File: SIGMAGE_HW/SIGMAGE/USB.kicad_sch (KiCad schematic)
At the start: 27 parts, among them J1 UJ31CHG2SMTTR, U13 ESDR0502NMUTBG, U9 FT2232HLTRAY

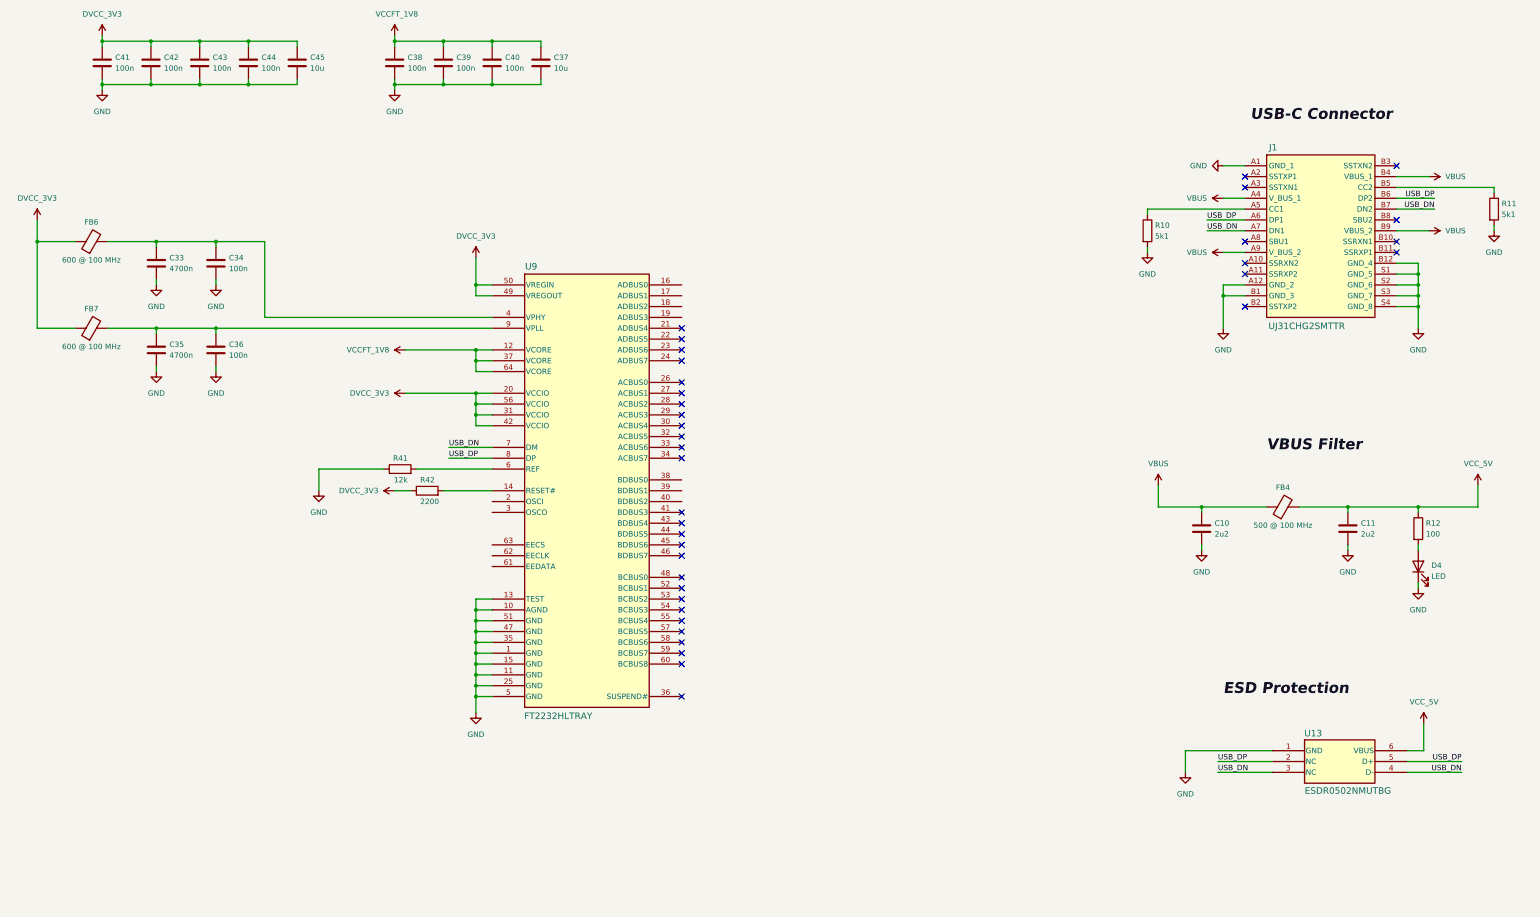
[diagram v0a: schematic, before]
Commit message: more USB stuff
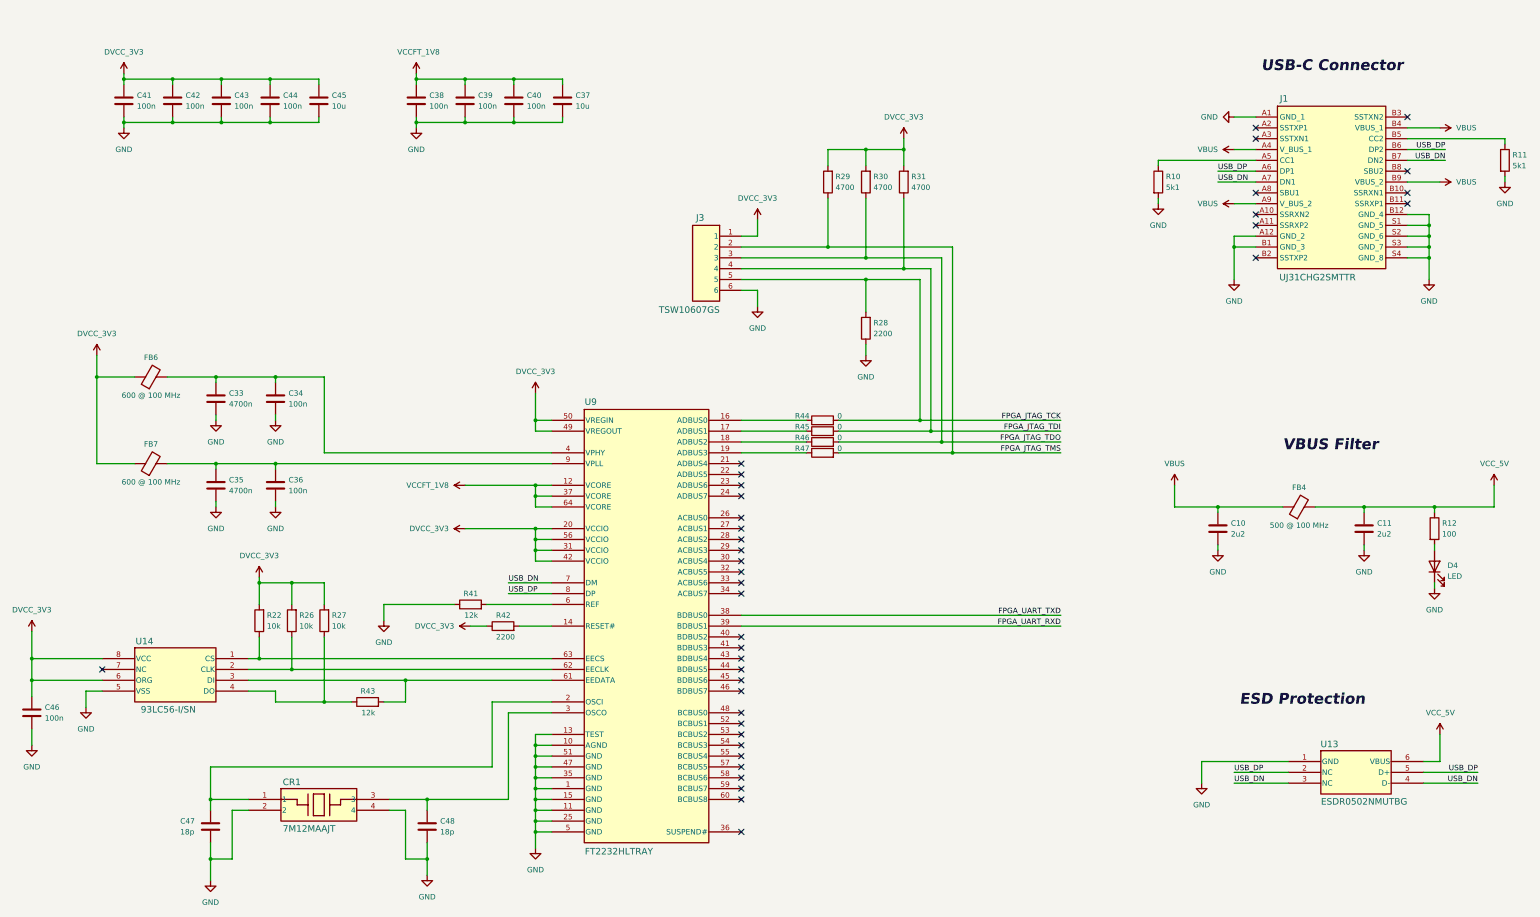
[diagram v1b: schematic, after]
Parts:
- added C46: 100n, Capacitor_SMD:C_0603_1608Metric, symbol Device:C
- added C47, C48: 18p, Capacitor_SMD:C_0603_1608Metric, symbol Device:C
- added CR1: 7M12MAAJT, SIGMAGE:7M12MAAJT, symbol SIGMAGE:7M12MAAJT
- added J3: TSW10607GS, SIGMAGE:TSW10607GS, symbol SIGMAGE:TSW10607GS
- added R22, R26, R27: 10k, Resistor_SMD:R_0603_1608Metric, symbol Device:R
- added R28: 2200, Resistor_SMD:R_0603_1608Metric, symbol Device:R
- added R29, R30, R31: 4700, Resistor_SMD:R_0603_1608Metric, symbol Device:R
- added R43: 12k, Resistor_SMD:R_0603_1608Metric, symbol Device:R
- added R44, R45, R46, R47: 0, Resistor_SMD:R_0603_1608Metric, symbol Device:R
- added U14: 93LC56-I/SN, SIGMAGE:93LC56ISN, symbol SIGMAGE:93LC56ISN
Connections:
- net DVCC_3V3: now also C46.1, J3.1, R22.2, R26.2, R27.2, R29.2, R30.2, R31.2, U14.6 (ORG), U14.8 (VCC)
- net GND: now also C46.2, C47.2, C48.2, CR1.2, CR1.4, J3.6, R28.1, U14.5 (VSS)
- net at U9.16 (ADBUS0): now also R44.1
- net at U9.17 (ADBUS1): now also R45.1
- net at U9.18 (ADBUS2): now also R46.1
- net at U9.19 (ADBUS3): now also R47.1
- net at U9.2 (OSCI): now also C47.1, CR1.1
- net at U9.3 (OSCO): now also C48.1, CR1.3
- net FPGA_UART_TXD: now reaches U9.38 (BDBUS0)
- net FPGA_UART_RXD: now reaches U9.39 (BDBUS1)
- net at U9.61 (EEDATA): now also R43.2, U14.3 (DI)
- net at U9.62 (EECLK): now also R26.1, U14.2 (CLK)
- net at U9.63 (EECS): now also R22.1, U14.1 (CS)
- new net: R27.1, R43.1, U14.4 (DO)
- new net FPGA_JTAG_TCK: J3.5, R28.2, R44.2
- new net FPGA_JTAG_TDI: J3.4, R31.1, R45.2
- new net FPGA_JTAG_TDO: J3.3, R30.1, R46.2
- new net FPGA_JTAG_TMS: J3.2, R29.1, R47.2
- no-connect marks 37 -> 39
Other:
- moved on the sheet: C10, C11, C33, C34, C35, C36, C37, C38, C39, C40, C41, C42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
